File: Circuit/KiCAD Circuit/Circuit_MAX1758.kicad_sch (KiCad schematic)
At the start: 63 parts, among them Q1 NMOS, Q2 NMOS, Q3 PMOS, U1 MAX1758, U2 ArduinoMKRZero, U3 MC7805ACTG, U4 BQ7692003PWR

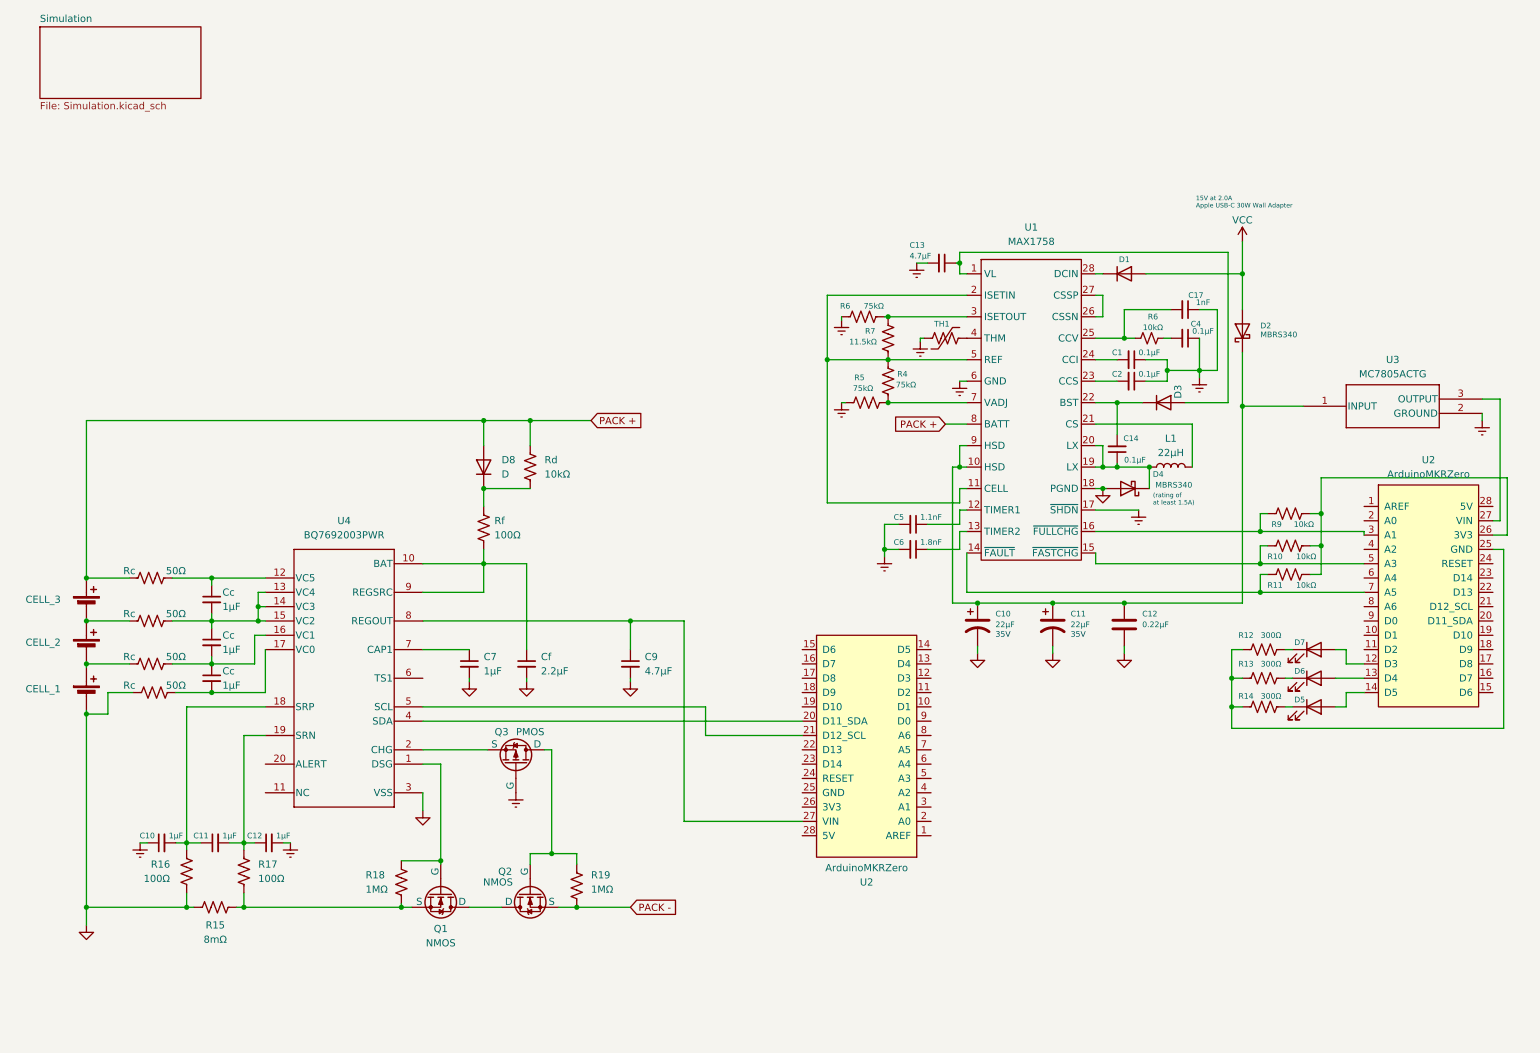
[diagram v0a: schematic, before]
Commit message: Backup
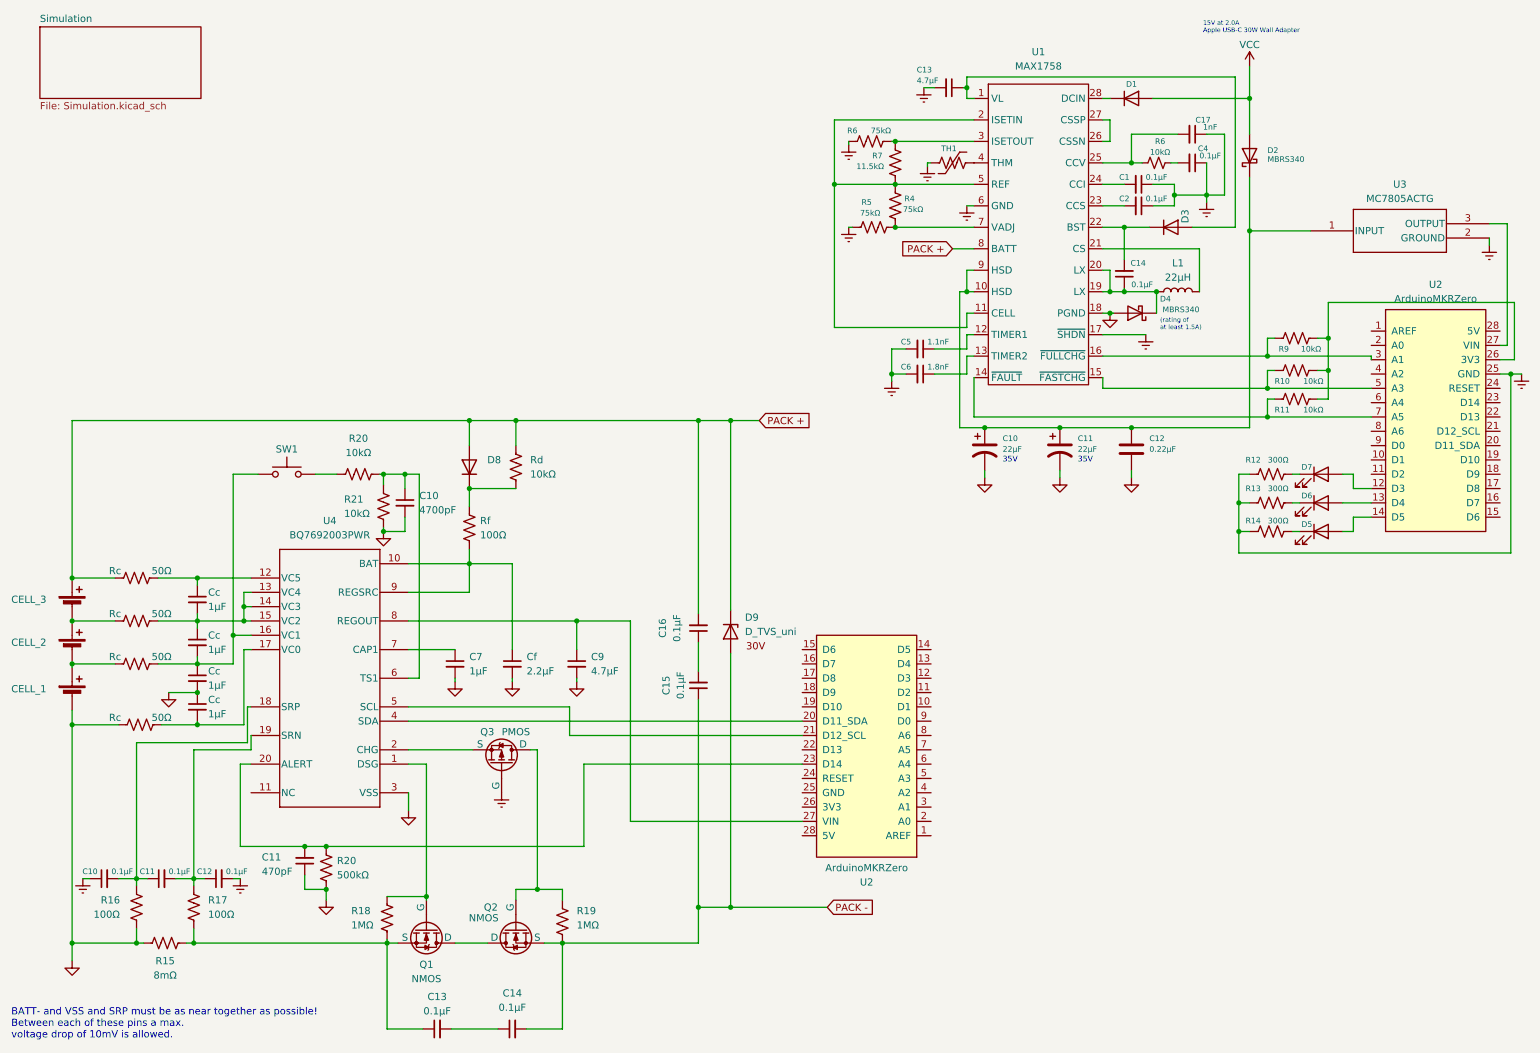
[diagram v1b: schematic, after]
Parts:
- added C10: 4700pF, symbol Device:C_Small
- added C11: 470pF, symbol Device:C_Small
- added C13, C14, C15, C16: 0.1μF, symbol Device:C_Small
- added Cc: 1μF, symbol Device:C_Small
- added D9: D_TVS_uni, symbol Device:D_Zener
- added R20: 500kΩ, symbol Device:R_US
- added R20, R21: 10kΩ, symbol Device:R_US
- added SW1: SW_Push, symbol Switch:SW_Push
- C10, C11, C12: value 1μF -> 0.1μF
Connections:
- net GND: now also Cc.2, C10.2, C11.1, Cc.1, R20.2, R21.2
- net GNDREF: now also R12.1, R13.1, R14.1, U2.25 (GND)
- net PACK +: now also C16.2, D9.1 (K)
- net PACK -: now also C14.2, C15.1, D9.2 (A)
- net at Cc.1, Cc.2, Rc.2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: now also SW1.1
- net at Rc.2, U4.17 (VC0): now also Cc.2; no longer Cc.2
- net at U4.20 (ALERT): now also U2.23 (D14), C11.2, R20.1
- net at U4.6 (TS1): now also C10.1, R20.2, R21.1
- net at Q1.3 (S), R15.2, R17.2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: now also C13.1
- new net: C13.2, C14.1
- new net: C15.2, C16.1
- new net: R20.1, SW1.2
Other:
- note added: "BATT- and VSS and SRP must be as near together as possible! Between each of these pins a max. voltage drop of 10mV is allowed."
- moved on the sheet: 50Ω, C1, C10, C11, C12, C13, C14, C17, C2, C4, C5, C6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
